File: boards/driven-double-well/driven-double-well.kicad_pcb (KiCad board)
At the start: 4 copper layers, 96.8 x 111.8 mm, 108 parts, among them J1 Conn_01x04, J2 Conn_01x03, J3 Conn_01x02, J4 Conn_01x02, J5 Conn_01x02, J6 Conn_01x03, J7 Conn_01x02, J8 Conn_01x02, Q1 BC560, Q2 BC560, Q3 BC560, Q4 BC560, Q5 BC560, U1 LM13700, U10 TL072, U11 TL072, U12 LM4040LP-10, U13 LM4040LP-10, U2 TL072, U3 MPY634KP, U4 MPY634KP, U5 TL072, U6 LM13700, U7 TL072, U8 LM334Z

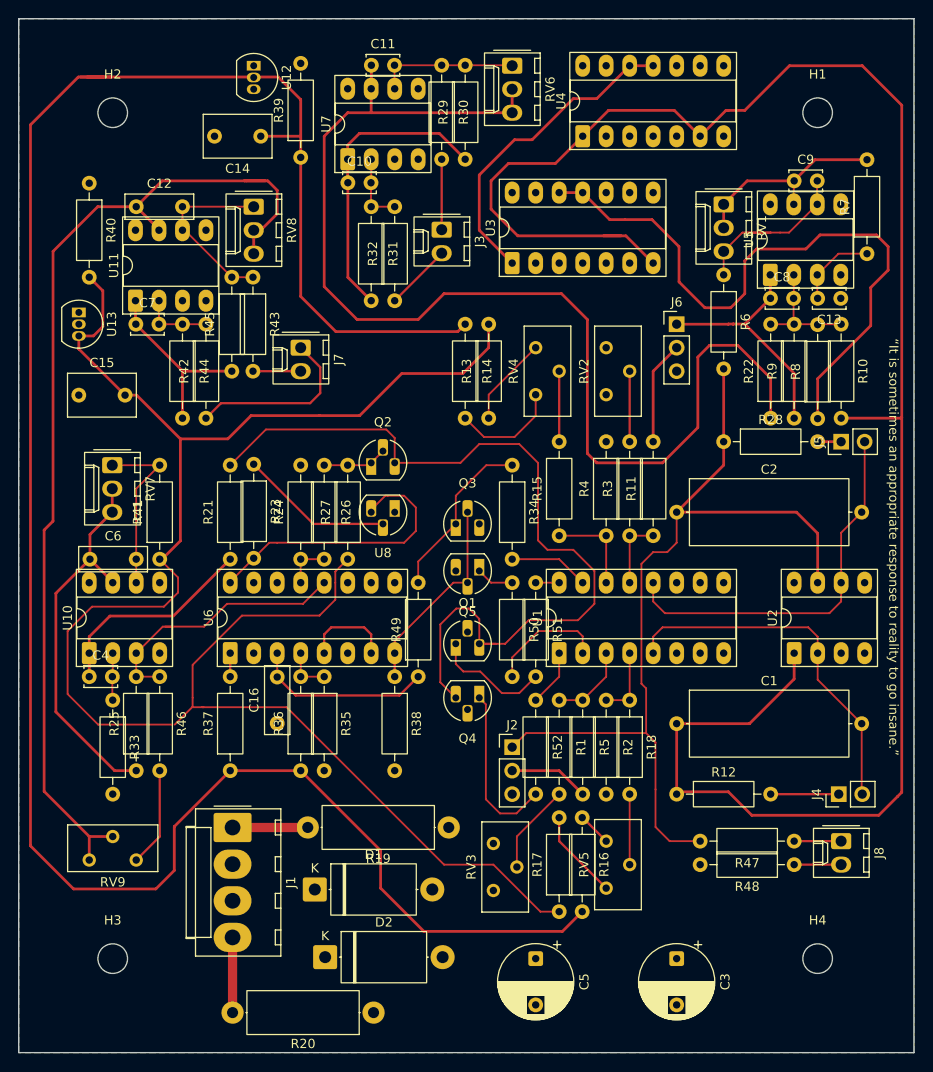
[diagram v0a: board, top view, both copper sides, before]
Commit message: Update driven double well board (#2)
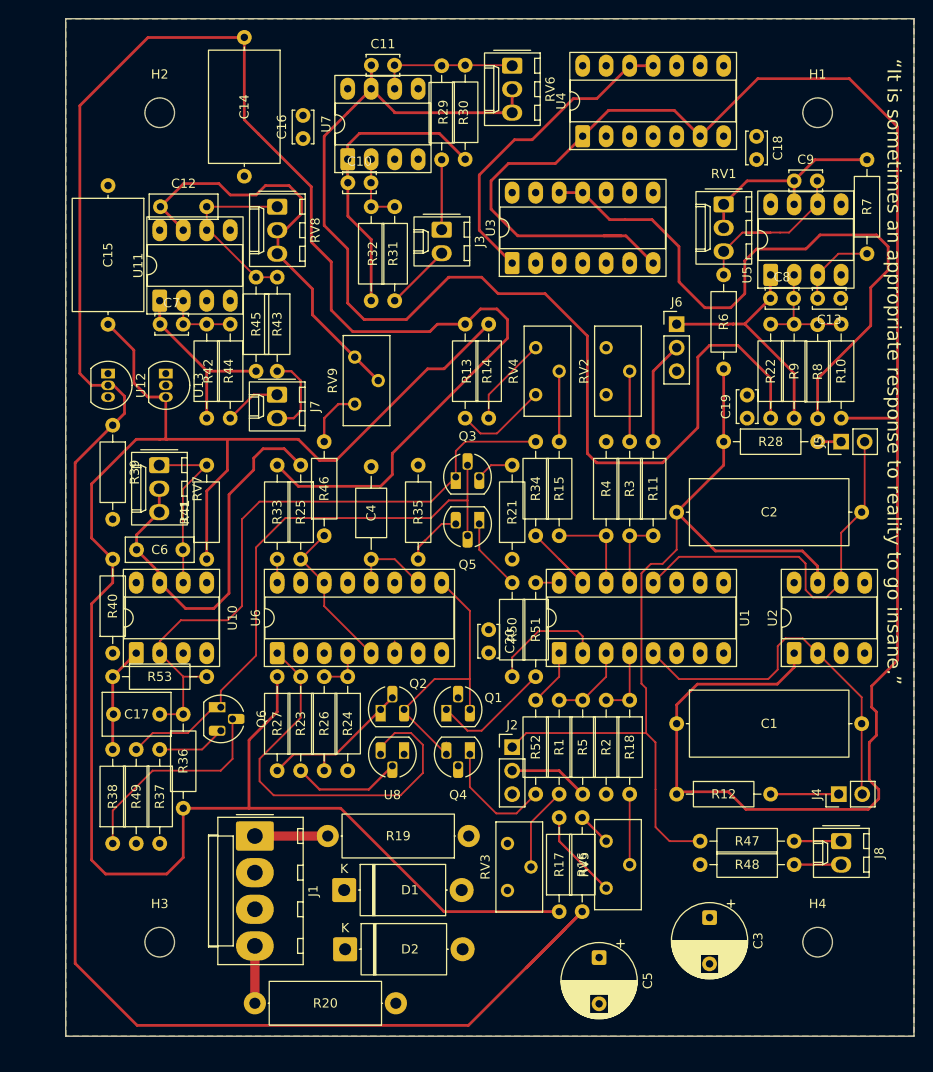
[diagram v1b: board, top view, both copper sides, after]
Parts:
- added C17: C, Capacitor_THT:C_Rect_L7.2mm_W4.5mm_P5.00mm_FKS2_FKP2_MKS2_MKP2, F.Cu at (45.8, 103.1)
- added C18: C, Capacitor_THT:C_Disc_D3.4mm_W2.1mm_P2.50mm, F.Cu at (115.3, 40.7)
- added C19: C, Capacitor_THT:C_Disc_D3.4mm_W2.1mm_P2.50mm, F.Cu at (114.3, 71.1)
- added C20: C, Capacitor_THT:C_Disc_D3.4mm_W2.1mm_P2.50mm, F.Cu at (86.4, 94.0)
- added Q6: BC550, Package_TO_SOT_THT:TO-92_HandSolder, F.Cu at (57.4, 102.4)
- added R53: 1meg, Resistor_THT:R_Axial_DIN0207_L6.3mm_D2.5mm_P10.16mm_Horizontal, F.Cu at (45.7, 99.1)
- C14, C15: footprint Capacitor_THT:C_Rect_L7.2mm_W4.5mm_P5.00mm_FKS2_FKP2_MKS2_MKP2 -> Capacitor_THT:C_Axial_L12.0mm_D7.5mm_P15.00mm_Horizontal
- C16: footprint Capacitor_THT:C_Rect_L7.2mm_W2.5mm_P5.00mm_FKS2_FKP2_MKS2_MKP2 -> Capacitor_THT:C_Disc_D3.4mm_W2.1mm_P2.50mm
- C4: footprint Capacitor_THT:C_Disc_D3.4mm_W2.1mm_P2.50mm -> Capacitor_THT:C_Axial_L5.1mm_D3.1mm_P10.00mm_Horizontal
- R21: value 10k -> 100
- R33: value 10k -> 1k
- R34, R35, R50: value 1k -> 100
- R37: value 100k -> 1k
- R38: value 1k -> 10k
- R49: value 1k -> 4.7k
- moved C16 63.3 mm to (66.3, 40.9)
- moved RV9 61.5 mm to (71.9, 64.5), turned to 90 degrees
- moved R40 50.9 mm to (45.7, 96.5), turned to 90 degrees
- moved R25 37.5 mm to (66.0, 76.2), turned to -90 degrees
- moved U12 36.8 mm to (45.2, 66.3)
- moved R38 35.4 mm to (45.7, 117.1), turned to 90 degrees
- moved R39 35.4 mm to (45.7, 71.9), turned to -90 degrees
- moved R23 33.5 mm to (66.0, 109.2), turned to 90 degrees
- moved C4 33.0 mm to (73.7, 86.4), turned to 90 degrees
- moved R26 33.0 mm to (68.6, 109.2), turned to 90 degrees
- moved R49 31.5 mm to (48.3, 106.9), turned to -90 degrees
- moved R33 31.0 mm to (63.5, 76.2)
- moved R21 30.5 mm to (88.9, 86.4)
- moved Q2 26.7 mm to (74.7, 102.6)
- moved U8 26.2 mm to (77.2, 107.4)
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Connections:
- C16 pad 2: Net-(U6C-+) -> +15V
- C4 pad 2: Net-(U10A--) -> GND
- Q3 pad 3: +15V -> Net-(Q3-E)
- Q5 pad 3: +15V -> Net-(Q5-E)
- R21 pad 1: Net-(C4-Pad1) -> +15V
- R21 pad 2: Net-(Q1-E) -> Net-(Q3-E)
- R24 pad 1: Net-(U6A--) -> Net-(U6C--)
- R25 pad 2: Net-(U10A-+) -> Net-(U6A-+)
- R26 pad 2: Net-(U6A--) -> Net-(U6C--)
- R33 pad 1: Net-(U10A--) -> /VREF_P10
- R33 pad 2: GND -> Net-(R33-Pad2)
- R35 pad 1: Net-(U6C--) -> +15V
- R35 pad 2: GND -> Net-(Q5-E)
- R36 pad 1: /VREF_P10 -> /VREF_N10
- R36 pad 2: Net-(U6C--) -> Net-(Q3-C)
- R37 pad 1: /VREF_P10 -> Net-(Q6-E)
- R37 pad 2: Net-(R37-Pad2) -> GND
- R38 pad 1: Net-(Q3-B) -> Net-(Q6-B)
- R38 pad 2: -15V -> Net-(C17-Pad1)
- R46 pad 1: Net-(U10A-+) -> Net-(U6A-+)
- R49 pad 1: Net-(U6C-+) -> Net-(Q3-B)
- R49 pad 2: Net-(Q3-C) -> +15V
- U10 pad 1: Net-(C4-Pad1) -> Net-(C17-Pad1)
- U10 pad 2: Net-(U10A--) -> Net-(Q3-C)
- U10 pad 3: Net-(U10A-+) -> GND
- U6 pad 1: Net-(R37-Pad2) -> Net-(R23-Pad2)
- U6 pad 10: unconnected-(U6-Pad10) -> Net-(C4-Pad1)
- U6 pad 12: Net-(U10A-+) -> Net-(C4-Pad1)
- U6 pad 13: Net-(U6A--) -> GND
- U6 pad 14: GND -> Net-(U6A-+)
- U6 pad 15: GND -> unconnected-(U6A-DIODE_BIAS-Pad15)
- U6 pad 16: Net-(R23-Pad2) -> Net-(R33-Pad2)
- U6 pad 2: unconnected-(U6C-DIODE_BIAS-Pad2) -> GND
- U6 pad 3: Net-(U6C-+) -> GND
- U6 pad 5: Net-(U6-Pad5) -> Net-(U6A-+)
- U6 pad 7: Net-(U6-Pad5) -> unconnected-(U6-Pad7)
- U6 pad 8: Net-(Q3-B) -> unconnected-(U6-Pad8)
- U6 pad 9: unconnected-(U6-Pad9) -> Net-(Q1-E)
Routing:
- net Net-(C12-Pad1): track 112.7 -> 46.2 mm
- net Net-(Q1-E): track 91.5 -> 30.9 mm
- net Net-(Q3-C): track 18.5 -> 70.7 mm
- net /VREF_P10: track 240.7 -> 281.4 mm
- net Net-(Q3-B): track 21.9 -> 62.5 mm
- net Net-(U10A-+): track 29.2 -> 0.00 mm
- net Net-(Q6-B): track 0.00 -> 23.1 mm
- net Net-(U6C-+): track 19.5 -> 0.00 mm
- net Net-(U6A-+): track 0.00 -> 17.9 mm
- net Net-(R23-Pad2): track 31.0 -> 45.6 mm
- net Net-(C4-Pad1): track 22.8 -> 9.43 mm
- net Net-(J7-Pin_1): track 19.3 -> 6.11 mm
- net Net-(C17-Pad1): track 0.00 -> 11.5 mm
- net Net-(Q2-B): track 6.98 -> 17.5 mm
- net Net-(U6-Pad5): track 9.78 -> 0.00 mm
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- added copper zone on F.Cu, net GND
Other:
- board size 96.8 x 111.8 mm -> 91.7 x 110 mm
